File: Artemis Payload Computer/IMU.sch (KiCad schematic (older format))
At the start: 1 part, among them U401 FXOS8700+FXAS21002

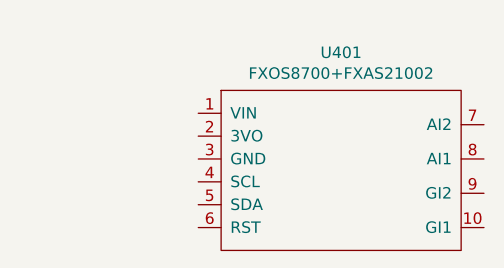
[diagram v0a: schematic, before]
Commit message: Shit
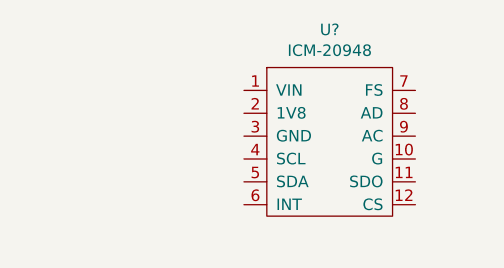
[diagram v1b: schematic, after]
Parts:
- removed U401: FXOS8700+FXAS21002, Artemis Payload Computer:IMU, symbol Artemis_Footprints:FXOS8700+FXAS21002
- added U?: ICM-20948, Artemis Payload Computer:ICM-20948, symbol Artemis_Footprints:ICM-20948
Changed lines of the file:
@@
 $EndDescr
 $Comp
-L Artemis_Footprints:FXOS8700+FXAS21002 U401
-U 1 1 603A9652
-P 6250 3450
-F 0 "U401" H 6275 3965 50  0000 C CNN
-F 1 "FXOS8700+FXAS21002" H 6275 3874 50  0000 C CNN
-F 2 "Artemis Payload Computer:IMU" H 6250 3450 50  0001 C CNN
-F 3 "" H 6250 3450 50  0001 C CNN
-	1    6250 3450
+L Artemis_Footprints:ICM-20948 U?
+U 1 1 60405DA7
+P 6200 3000
+F 0 "U?" H 6225 3165 50  0000 C CNN
+F 1 "ICM-20948" H 6225 3074 50  0000 C CNN
+F 2 "Artemis Payload Computer:ICM-20948" H 6200 3000 50  0001 C CNN
+F 3 "" H 6200 3000 50  0001 C CNN
+	1    6200 3000
 	1    0    0    -1
 $EndComp

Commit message: ready for testing...
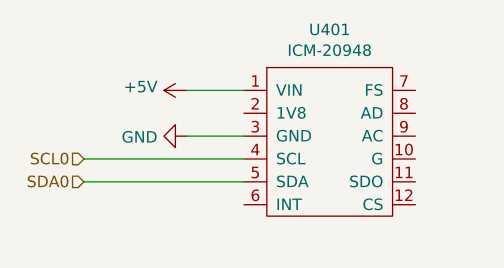
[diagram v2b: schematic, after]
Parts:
- gave numbers to parts that had none: 1
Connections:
- net +5V: now reaches U401.1 (VIN)
- net GND: now reaches U401.3 (GND)
- net SCL0: now reaches U401.4 (SCL)
- net SDA0: now reaches U401.5 (SDA)
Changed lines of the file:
@@
 $EndDescr
 $Comp
-L Artemis_Footprints:ICM-20948 U?
+L Artemis_Footprints:ICM-20948 U401
 U 1 1 60405DA7
 P 6200 3000
-F 0 "U?" H 6225 3165 50  0000 C CNN
+F 0 "U401" H 6225 3165 50  0000 C CNN
 F 1 "ICM-20948" H 6225 3074 50  0000 C CNN
 F 2 "Artemis Payload Computer:ICM-20948" H 6200 3000 50  0001 C CNN
@@
 	1    0    0    -1
 $EndComp
+$Comp
+L power:+5V #PWR0109
+U 1 1 604076E6
+P 5600 3100
+F 0 "#PWR0109" H 5600 2950 50  0001 C CNN
+F 1 "+5V" V 5615 3228 50  0000 L CNN
+F 2 "" H 5600 3100 50  0001 C CNN
+F 3 "" H 5600 3100 50  0001 C CNN
+	1    5600 3100
+	0    -1   -1   0
+$EndComp
+$Comp
+L power:GND #PWR0110
+U 1 1 604079B0
+P 5600 3300
+F 0 "#PWR0110" H 5600 3050 50  0001 C CNN
+F 1 "GND" V 5605 3172 50  0000 R CNN
+F 2 "" H 5600 3300 50  0001 C CNN
+F 3 "" H 5600 3300 50  0001 C CNN
+	1    5600 3300
+	0    1    1    0
+$EndComp
+Wire Wire Line
+	5600 3100 5850 3100
+Wire Wire Line
+	5850 3300 5600 3300
+Text HLabel 5150 3400 0    50   Input ~ 0
+SCL0
+Text HLabel 5150 3500 0    50   Input ~ 0
+SDA0
+Wire Wire Line
+	5850 3400 5150 3400
+Wire Wire Line
+	5150 3500 5850 3500
 $EndSCHEMATC
